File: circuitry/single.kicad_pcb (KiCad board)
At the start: 2 copper layers, 88 x 43.6 mm, 38 parts, among them J1 Conn_01x02, J2 Conn_01x03, P1 Touch_Pad, SW1 SW_Push, U1 MIC5225-5.0YM5, U2 ATtiny402-SS, U3 74LVC2GU04, Y1 16MHz

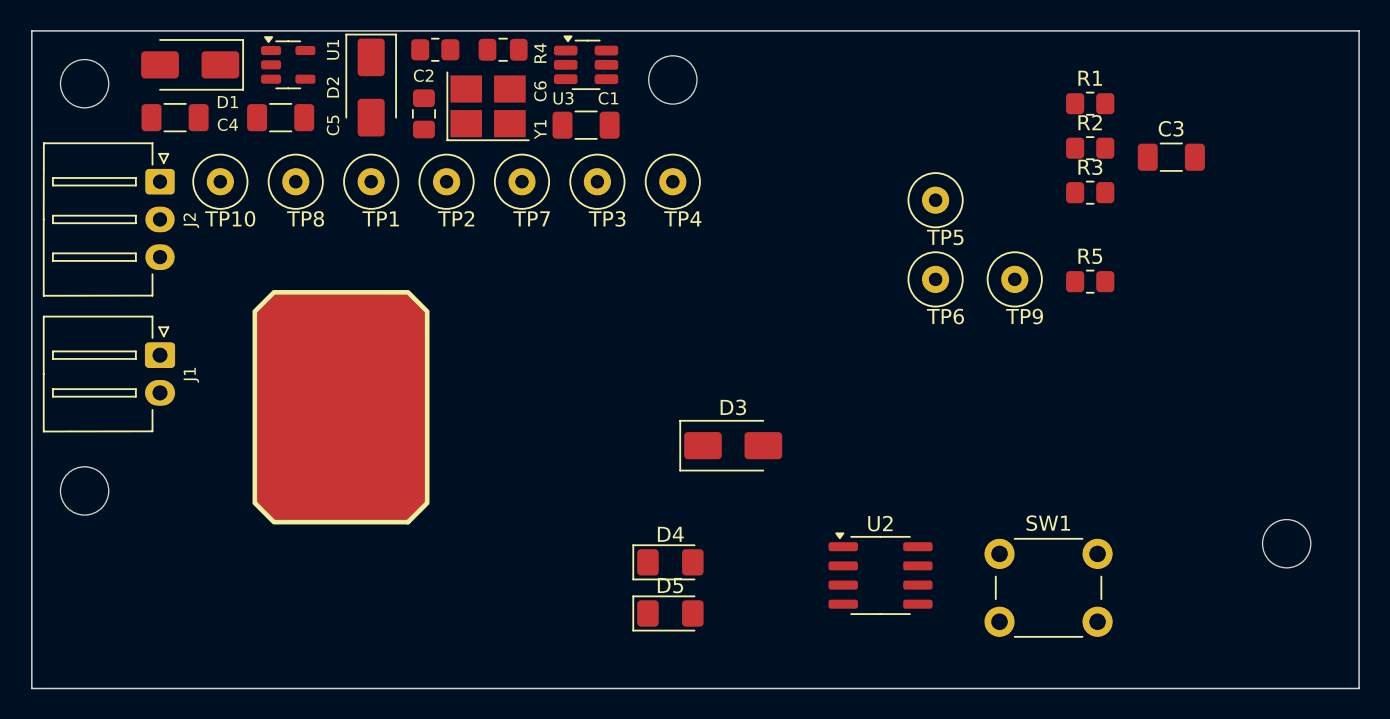
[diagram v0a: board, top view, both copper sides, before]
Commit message: Completed schematic and layout.
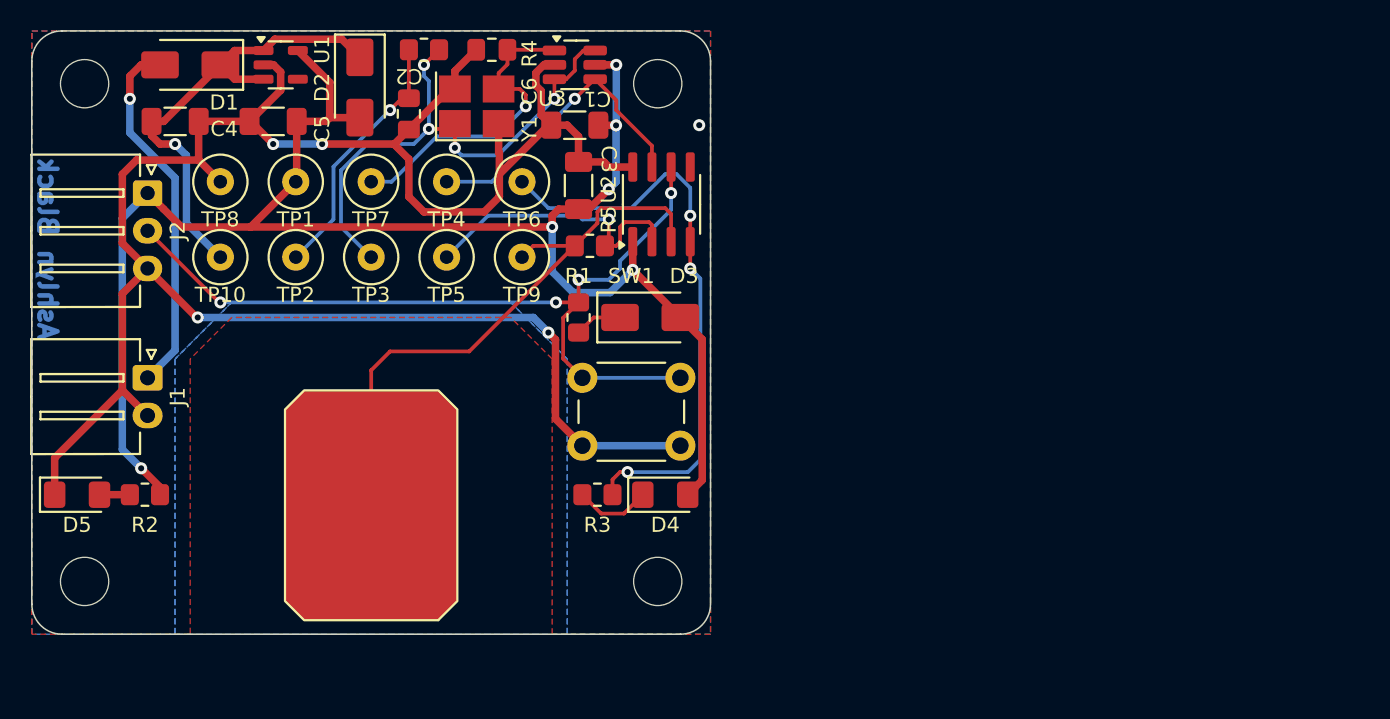
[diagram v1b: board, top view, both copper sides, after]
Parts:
- removed the REF** at (122.5, 120.5)
- removed the REF** at (202.2, 124.0)
- removed the REF** at (161.5, 93.2)
- added REF**: MountingHole_3.2mm_M3_DIN965, MountingHole:MountingHole_3.2mm_M3_DIN965, F.Cu at (160.5, 126.5)
- added REF**: MountingHole_3.2mm_M3_DIN965, MountingHole:MountingHole_3.2mm_M3_DIN965, F.Cu at (122.5, 126.5)
- added REF**: MountingHole_3.2mm_M3_DIN965, MountingHole:MountingHole_3.2mm_M3_DIN965, F.Cu at (160.5, 93.5)
- moved R2 66.8 mm to (126.5, 120.8), turned to 180 degrees
- moved D5 40.1 mm to (122.0, 120.8)
- moved C3 39.3 mm to (155.2, 100.2), turned to 90 degrees
- moved R3 38.3 mm to (156.5, 120.8), turned to 180 degrees
- moved R1 36.8 mm to (155.2, 109.0), turned to 90 degrees
- moved R5 33.3 mm to (156.0, 104.2), turned to 180 degrees
- moved TP9 32.7 mm to (151.5, 105.0)
- moved TP5 32.6 mm to (146.5, 105.0)
- moved U2 28.6 mm to (160.8, 101.5), turned to 90 degrees
- moved TP6 28.2 mm to (151.5, 100.0)
- moved SW1 22.3 mm to (162.0, 117.5), turned to 180 degrees
- moved TP3 15.8 mm to (141.5, 105.0)
- moved TP4 15.0 mm to (146.5, 100.0)
- moved TP2 11.2 mm to (136.5, 105.0)
- moved D3 10.1 mm to (160.0, 109.0)
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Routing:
- net GND: track 0.00 -> 141.3 mm, vias 0 -> 5
- net VCC: track 0.00 -> 112.2 mm, vias 0 -> 6
- net ~{RST}: track 0.00 -> 55.7 mm, vias 0 -> 4
- net Net-(U2-PA7): track 0.00 -> 40.8 mm
- net Net-(U2-PA1): track 0.00 -> 38.9 mm, vias 0 -> 3
- net Net-(U3-A2): track 0.00 -> 36.5 mm, vias 0 -> 4
- net +BATT: track 0.00 -> 31.3 mm, vias 0 -> 1
- net Net-(D1-A): track 0.00 -> 24.3 mm, vias 0 -> 1
- net Net-(U3-A1): track 0.00 -> 21.5 mm, vias 0 -> 1
- net MCLK: track 0.00 -> 20.1 mm, vias 0 -> 1
- net Net-(U2-PA6): track 0.00 -> 19.6 mm, vias 0 -> 1
- net Net-(C2-Pad2): track 0.00 -> 17.1 mm, vias 0 -> 1
- net Net-(D4-K): track 0.00 -> 5.05 mm
- net Net-(D3-K): track 0.00 -> 3.16 mm
- net Net-(D5-A): track 0.00 -> 2.01 mm
- added copper zone on B.Cu, net GND
- added copper zone on F.Cu, net GND
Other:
- board size 88 x 43.6 mm -> 45 x 40 mm
